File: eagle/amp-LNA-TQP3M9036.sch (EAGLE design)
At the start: 13 parts, among them U1 TQP3M9036, X1 SMA, X2 SMA

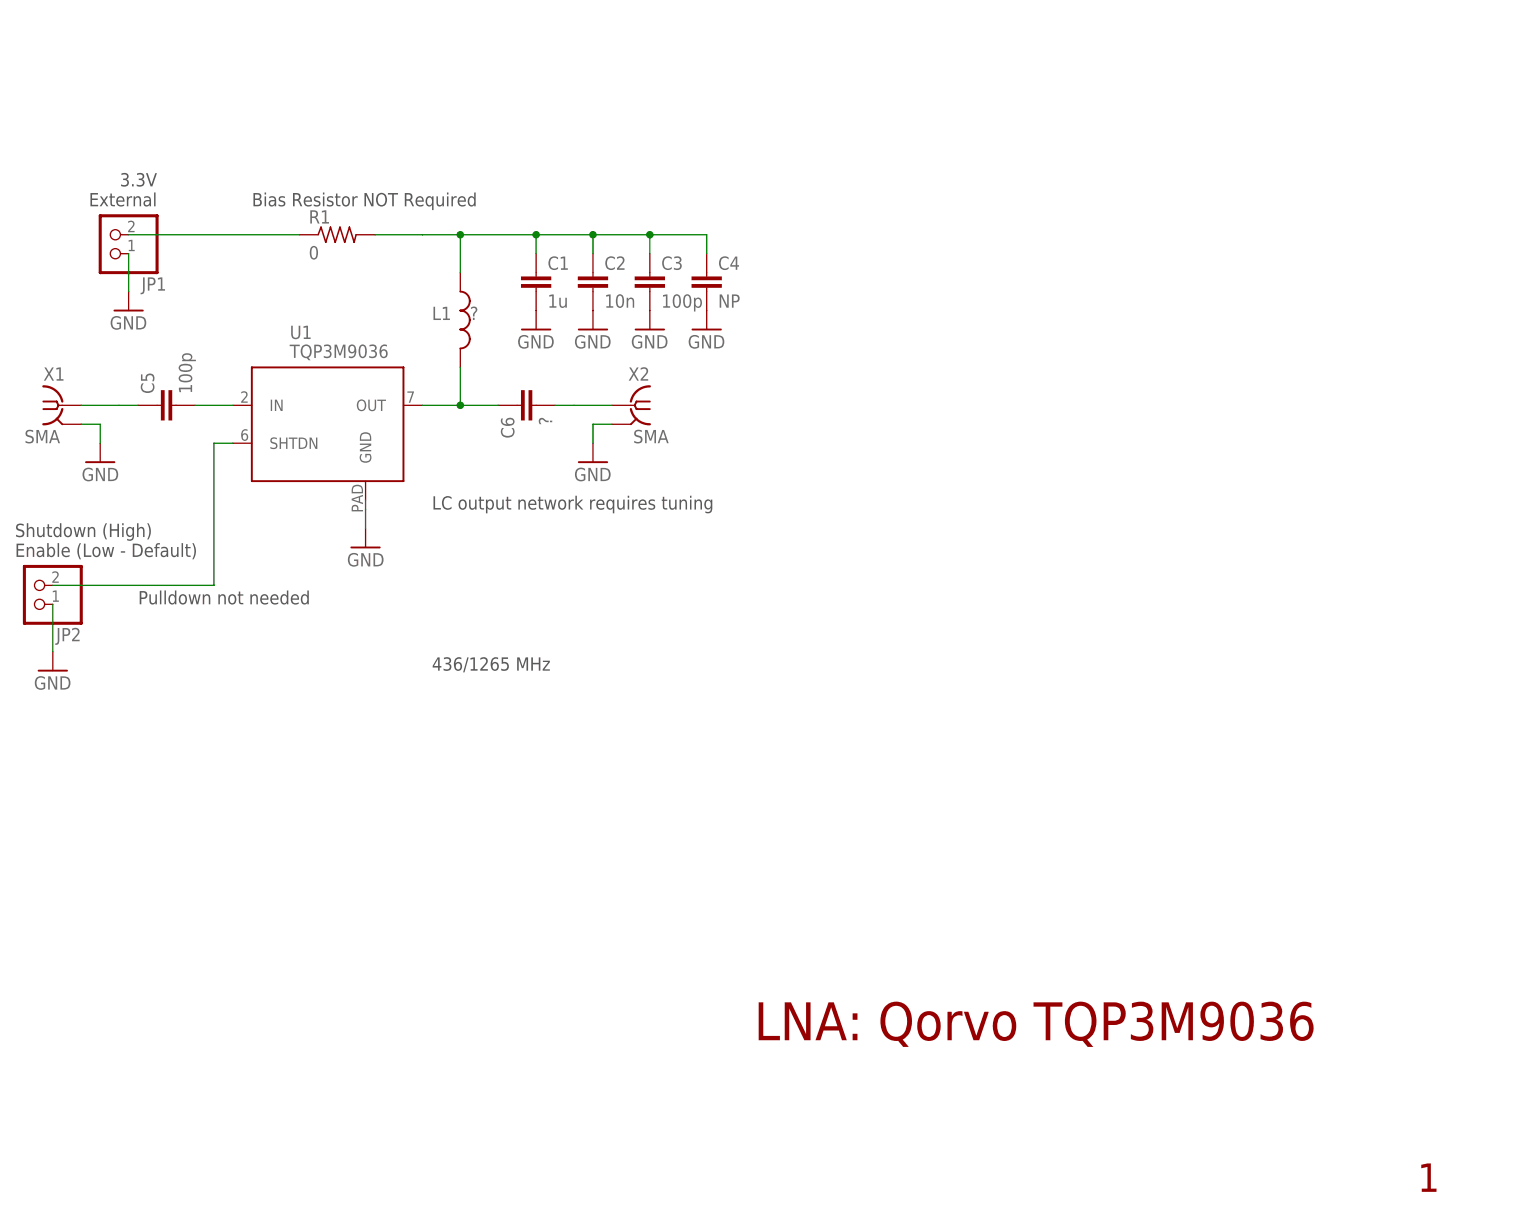
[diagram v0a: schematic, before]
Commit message: Add features and minor fixes
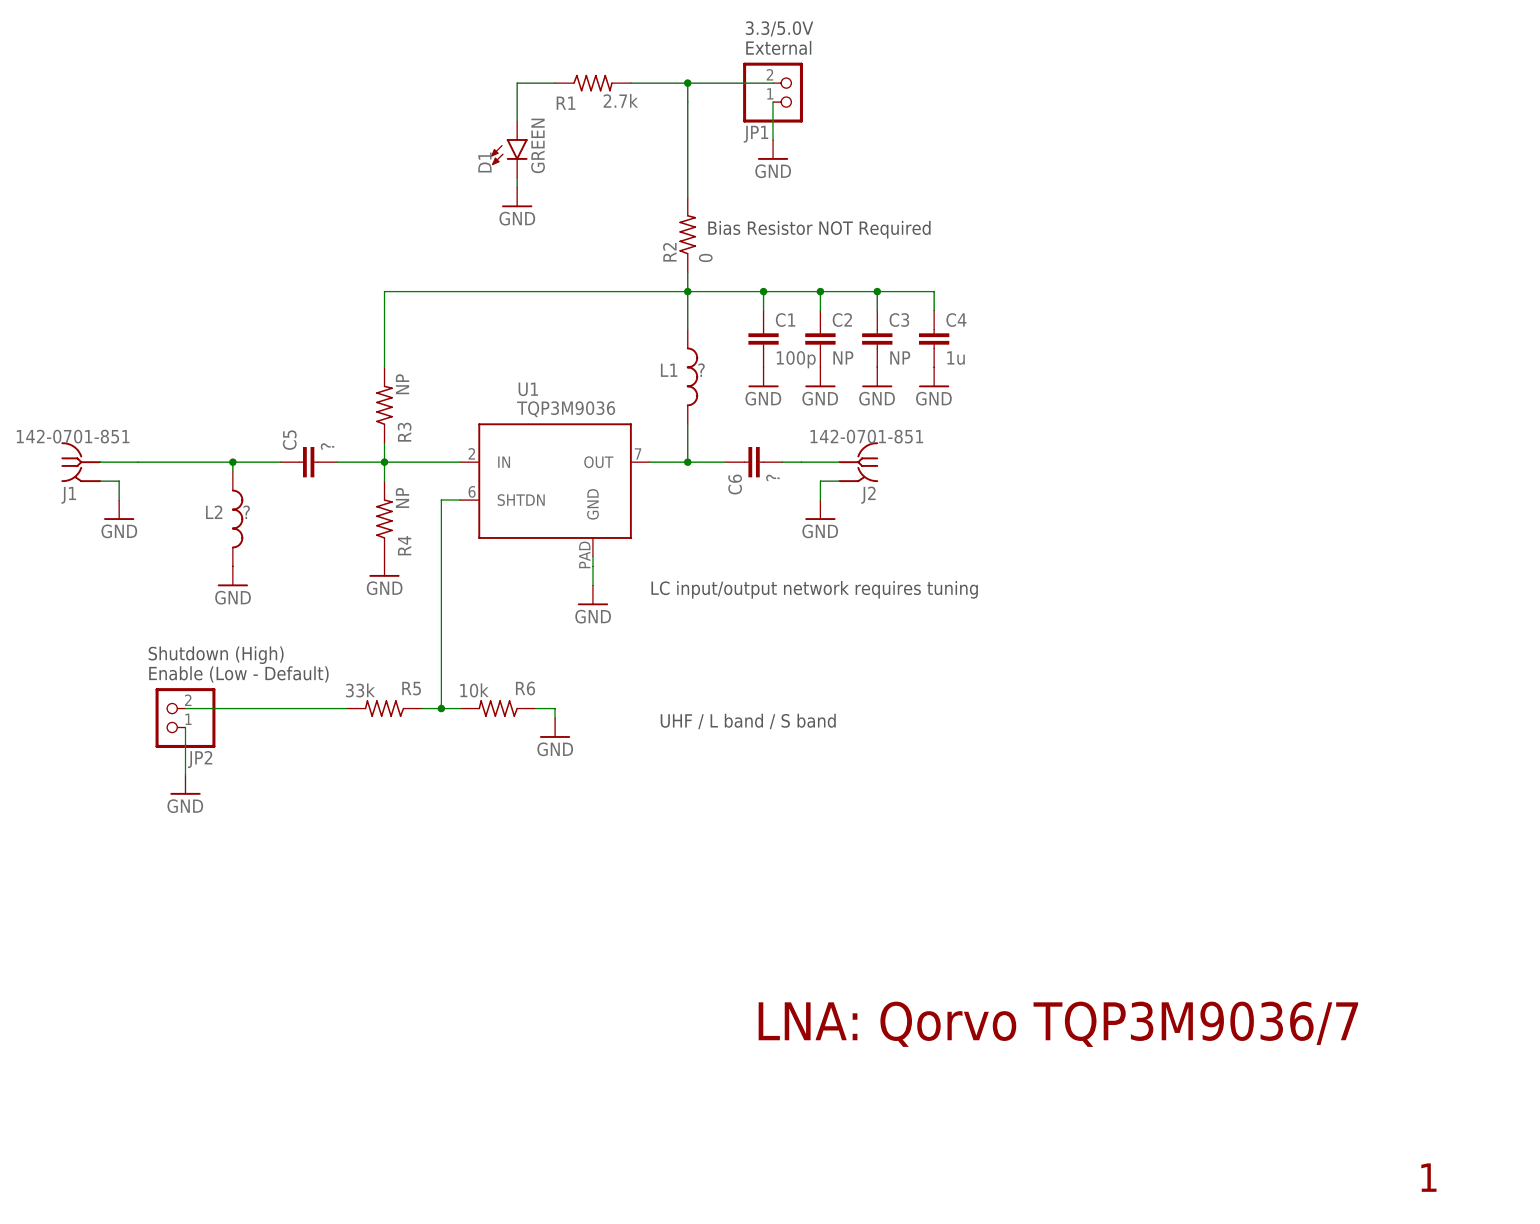
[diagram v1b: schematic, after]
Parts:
- removed X1, X2: SMA, con-coax:SMA-142-0701-801/806
- added D1: GREEN, SparkFun-LED:LED-GREEN0603
- added J1, J2: 142-0701-851, J-Cinch-142-0701-851-SMA-end-launch:142-0701-851
- added L2: ?, oresat-rcl:L-US0402-B-NOSILK
- added R2: 0, oresat-rcl:R-US_0805-B-NOSILK
- added R3, R4: NP, oresat-rcl:R-US_0402-B-NOSILK
- added R5: 33k, oresat-rcl:R-US_0603-B-NOSILK
- added R6: 10k, oresat-rcl:R-US_0603-B-NOSILK
- C1: value 1u -> 100p
- C2: value 10n -> NP
- C3: value 100p -> NP
- C4: value NP -> 1u
- C5: value 100p -> ?
- L1: device oresat-rcl:L-US0805-B-NOSILK -> oresat-rcl:L-US0603-B-NOSILK
- R1: value 0 -> 2.7k; device oresat-rcl:R-US_0805-B-NOSILK -> oresat-rcl:R-US_0603-B-NOSILK
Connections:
- new net N$21: D1.A, R1.1
- new net N$3: JP2.2, R5.2
- net GND: now also D1.C, J1.GND, J2.GND, L2.2, R4.1, R6.1; no longer X1.2, X2.2
- net N$1: now also R1.2, R2.2; no longer R1.1
- net N$2: now also R5.1, R6.2; no longer JP2.2
- net N$32: now also R3.1, R4.2
- net N$34: now also J2.RF; no longer X2.1
- net N$39: now also J1.RF, L2.1; no longer X1.1
- net N$47: now also R2.1, R3.2; no longer R1.2
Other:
- note added: "3.3/5.0V External"
- note added: "LC input/output network requires tuning"
- note added: "LNA: Qorvo TQP3M9036/7"
- note added: "UHF / L band / S band"
- note removed: "3.3V External"
- note removed: "436/1265 MHz"
- note removed: "LC output network requires tuning"
- note removed: "LNA: Qorvo TQP3M9036"
- note removed: "Pulldown not needed"
- moved on the sheet: C1, C2, C3, C4, C5, C6, JP1, JP2, L1, R1, U1
